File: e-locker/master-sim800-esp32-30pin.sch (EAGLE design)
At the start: 57 parts, among them T1 BC847, T2 BC847, T3 BC847, T4 BC847, U1 AT24C128C-SSHM-T, X1 JST-XH-02-PIN-LONG-PAD, X10 JST-XH-05-PIN-LONG-PAD, X11 JST-XH-02-PIN-LONG-PAD, X12 JST-XH-02-PIN-LONG-PAD, X13 JST-XH-02-PIN-LONG-PAD, X2 JST-XH-02-PIN-LONG-PAD, X3 JST-XH-02-PIN-LONG-PAD, X4 JST-XH-02-PIN-LONG-PAD, X5 JST-XH-02-PIN-LONG-PAD, X6 JST-XH-02-PIN-LONG-PAD, X7 JST-XH-04-PIN-LONG-PAD, X8 JST-XH-05-PIN-LONG-PAD, X9 JST-XH-05-PIN-LONG-PAD

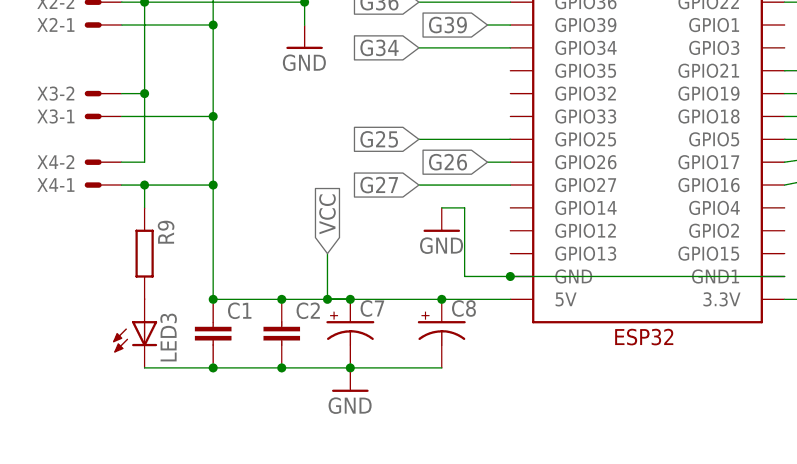
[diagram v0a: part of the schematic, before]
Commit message: QR code reader header
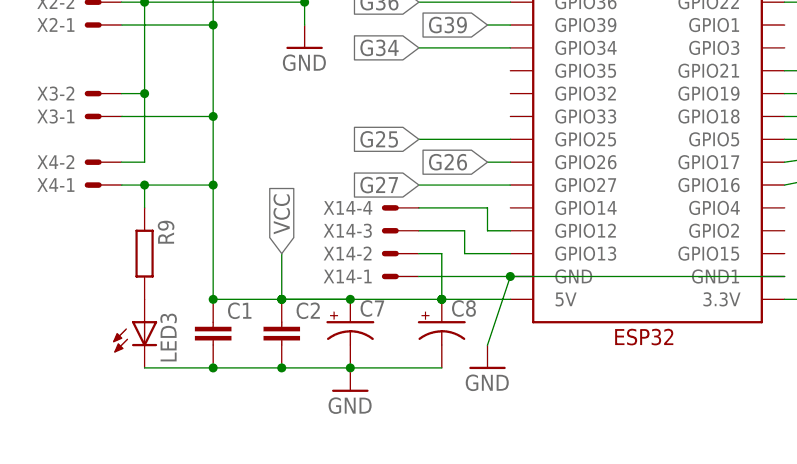
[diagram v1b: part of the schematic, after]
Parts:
- added X14: JST-XH-04-PIN-LONG-PAD, Rembrandt Electronics - JST XH Connectors v1-0:JST-XH-04-PIN-LONG-PAD
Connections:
- new net N$30: U$1.GPIO13, X14-3.S
- new net N$31: U$1.GPIO12, X14-4.S
- net GND: now also X14-1.S
- net VCC: now also X14-2.S
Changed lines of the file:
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@@
 <part name="R15" library="eagle-ltspice" library_urn="urn:adsk.eagle:library:217" deviceset="R" device="R1206" package3d_urn="urn:adsk.eagle:package:13301/1" value="5.6k"/>
 <part name="R16" library="eagle-ltspice" library_urn="urn:adsk.eagle:library:217" deviceset="R" device="R1206" package3d_urn="urn:adsk.eagle:package:13301/1" value="5.6k"/>
+<part name="X14" library="Rembrandt Electronics - JST XH Connectors v1-0" deviceset="JST-XH-04-PIN" device="-LONG-PAD"/>
 </parts>
 <sheets>
@@
 <attribute name="VALUE" x="104.14" y="33.02" size="1.778" layer="96"/>
 </instance>
-<instance part="GND2" gate="1" x="15.24" y="43.18" smashed="yes">
-<attribute name="VALUE" x="12.7" y="40.64" size="1.778" layer="96"/>
+<instance part="GND2" gate="1" x="20.32" y="27.94" smashed="yes">
+<attribute name="VALUE" x="17.78" y="25.4" size="1.778" layer="96"/>
 </instance>
 <instance part="GND3" gate="1" x="124.46" y="22.86" smashed="yes">
@@
 <attribute name="NAME" x="90.17" y="118.3386" size="1.778" layer="95"/>
 <attribute name="VALUE" x="90.17" y="113.538" size="1.778" layer="96"/>
+</instance>
+<instance part="X14" gate="-1" x="10.16" y="38.1" smashed="yes" rot="R180">
+<attribute name="NAME" x="7.62" y="38.862" size="1.524" layer="95" rot="R180"/>
+</instance>
+<instance part="X14" gate="-2" x="10.16" y="40.64" smashed="yes" rot="R180">
+<attribute name="NAME" x="7.62" y="41.402" size="1.524" layer="95" rot="R180"/>
+</instance>
+<instance part="X14" gate="-3" x="10.16" y="43.18" smashed="yes" rot="R180">
+<attribute name="NAME" x="7.62" y="43.942" size="1.524" layer="95" rot="R180"/>
+</instance>
+<instance part="X14" gate="-4" x="10.16" y="45.72" smashed="yes" rot="R180">
+<attribute name="NAME" x="7.62" y="46.482" size="1.524" layer="95" rot="R180"/>
 </instance>
 </instances>
@@
 <wire x1="-10.16" y1="48.26" x2="-10.16" y2="35.56" width="0.1524" layer="91"/>
 <wire x1="-10.16" y1="35.56" x2="-2.54" y2="35.56" width="0.1524" layer="91"/>
-<wire x1="-2.54" y1="35.56" x2="5.08" y2="35.56" width="0.1524" layer="91"/>
-<wire x1="5.08" y1="35.56" x2="2.54" y2="35.56" width="0.1524" layer="91"/>
-<wire x1="2.54" y1="35.56" x2="15.24" y2="35.56" width="0.1524" layer="91"/>
+<wire x1="5.08" y1="35.56" x2="-2.54" y2="35.56" width="0.1524" layer="91"/>
+<wire x1="-2.54" y1="35.56" x2="15.24" y2="35.56" width="0.1524" layer="91"/>
 <wire x1="15.24" y1="35.56" x2="22.86" y2="35.56" width="0.1524" layer="91"/>
-<wire x1="2.54" y1="35.56" x2="2.54" y2="40.64" width="0.1524" layer="91"/>
-<junction x="2.54" y="35.56"/>
-<label x="2.54" y="40.64" size="1.778" layer="95" rot="R90" xref="yes"/>
+<wire x1="-2.54" y1="35.56" x2="-2.54" y2="40.64" width="0.1524" layer="91"/>
+<junction x="-2.54" y="35.56"/>
+<label x="-2.54" y="40.64" size="1.778" layer="95" rot="R90" xref="yes"/>
 <pinref part="X2" gate="-1" pin="S"/>
 <wire x1="-20.32" y1="66.04" x2="-10.16" y2="66.04" width="0.1524" layer="91"/>
@@
 <wire x1="-17.78" y1="45.72" x2="-17.78" y2="48.26" width="0.1524" layer="91"/>
 <junction x="-17.78" y="48.26"/>
+<pinref part="X14" gate="-2" pin="S"/>
+<wire x1="12.7" y1="40.64" x2="15.24" y2="40.64" width="0.1524" layer="91"/>
+<wire x1="15.24" y1="40.64" x2="15.24" y2="35.56" width="0.1524" layer="91"/>
+<junction x="15.24" y="35.56"/>
 </segment>
 </net>
@@
 <segment>
 <pinref part="U$1" gate="G$1" pin="GND"/>
-<wire x1="22.86" y1="38.1" x2="17.78" y2="38.1" width="0.1524" layer="91"/>
-<wire x1="17.78" y1="38.1" x2="17.78" y2="45.72" width="0.1524" layer="91"/>
+<wire x1="22.86" y1="38.1" x2="20.32" y2="30.48" width="0.1524" layer="91"/>
 <pinref part="GND2" gate="1" pin="GND"/>
-<wire x1="17.78" y1="45.72" x2="15.24" y2="45.72" width="0.1524" layer="91"/>
 <pinref part="U$1" gate="G$1" pin="GND1"/>
 <wire x1="53.34" y1="38.1" x2="22.86" y2="38.1" width="0.1524" layer="91"/>
 <junction x="22.86" y="38.1"/>
+<pinref part="X14" gate="-1" pin="S"/>
+<wire x1="12.7" y1="38.1" x2="22.86" y2="38.1" width="0.1524" layer="91"/>
 </segment>
 </net>
@@
 </segment>
 </net>
+<net name="N$30" class="0">
+<segment>
+<pinref part="U$1" gate="G$1" pin="GPIO13"/>
+<wire x1="22.86" y1="40.64" x2="17.78" y2="40.64" width="0.1524" layer="91"/>
+<wire x1="17.78" y1="40.64" x2="17.78" y2="43.18" width="0.1524" layer="91"/>
+<pinref part="X14" gate="-3" pin="S"/>
+<wire x1="17.78" y1="43.18" x2="12.7" y2="43.18" width="0.1524" layer="91"/>
+</segment>
+</net>
+<net name="N$31" class="0">
+<segment>
+<pinref part="U$1" gate="G$1" pin="GPIO12"/>
+<wire x1="22.86" y1="43.18" x2="20.32" y2="43.18" width="0.1524" layer="91"/>
+<wire x1="20.32" y1="43.18" x2="20.32" y2="45.72" width="0.1524" layer="91"/>
+<pinref part="X14" gate="-4" pin="S"/>
+<wire x1="20.32" y1="45.72" x2="12.7" y2="45.72" width="0.1524" layer="91"/>
+</segment>
+</net>

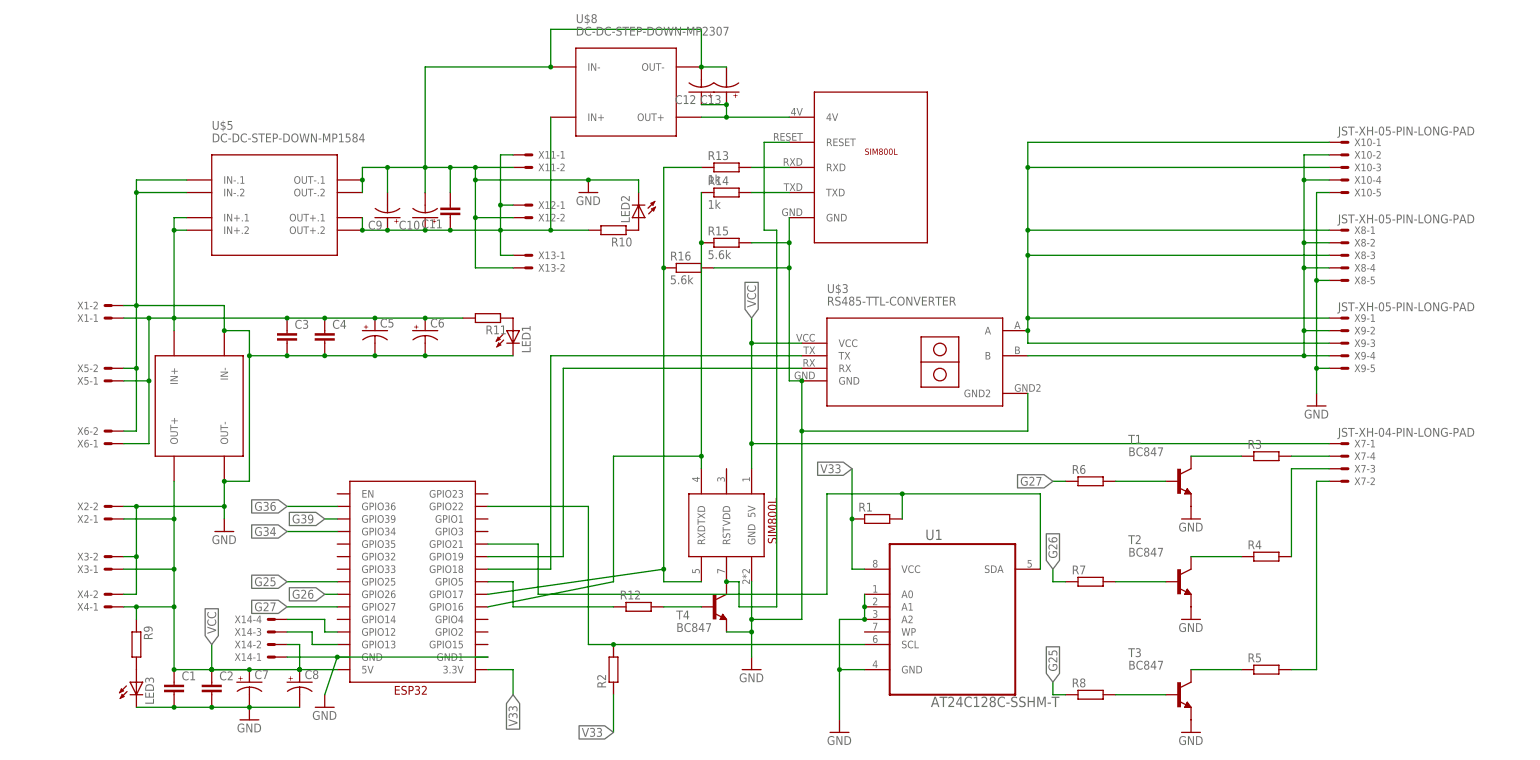
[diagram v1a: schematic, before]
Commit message: v1.7
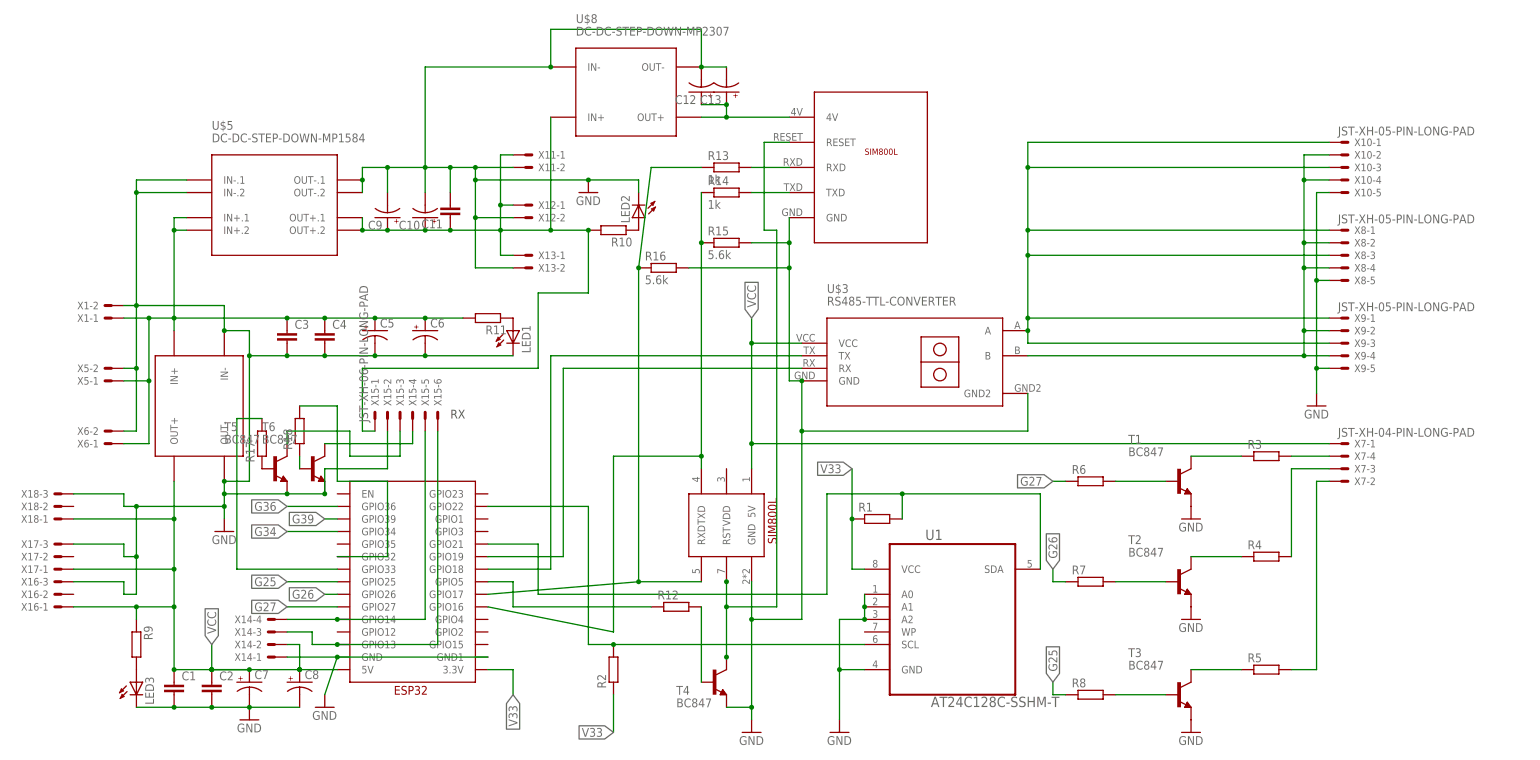
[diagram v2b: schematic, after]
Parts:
- removed X2, X3, X4: JST-XH-02-PIN-LONG-PAD, Rembrandt Electronics - JST XH Connectors v1-0:JST-XH-02-PIN-LONG-PAD
- added R17, R18: (no value), eagle-ltspice:RR1206
- added T5, T6: BC847, transistor:BC847
- added X15: JST-XH-06-PIN-LONG-PAD, Rembrandt Electronics - JST XH Connectors v1-0:JST-XH-06-PIN-LONG-PAD
- added X16, X17, X18: JST-XH-03-PIN-LONG-PAD, Rembrandt Electronics - JST XH Connectors v1-0:JST-XH-03-PIN-LONG-PAD
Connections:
- new net N$32: R17.1, T5.B
- new net N$33: R18.1, T6.B
- new net N$34: R18.2, U$1.GPIO32
- new net N$35: T6.C, X15-4.S
- new net N$36: T5.C, X15-3.S
- new net N$37: R17.2, U$1.GPIO33
- net GND: now also T5.E, T6.E, X15-2.S, X16-3.S, X17-3.S, X18-3.S; no longer X2-2.S, X3-2.S, X4-2.S
- net N$23: now also X15-1.S
- net N$30: now also X15-6.S
- net N$31: now also U$1.GPIO14, X15-5.S; no longer U$1.GPIO12
- net VCC: now also X16-1.S, X17-1.S, X18-1.S; no longer X2-1.S, X3-1.S, X4-1.S
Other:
- note added: "RX"
- moved on the sheet: R12, R16, T4
